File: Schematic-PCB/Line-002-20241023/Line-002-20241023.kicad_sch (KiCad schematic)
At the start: 208 parts

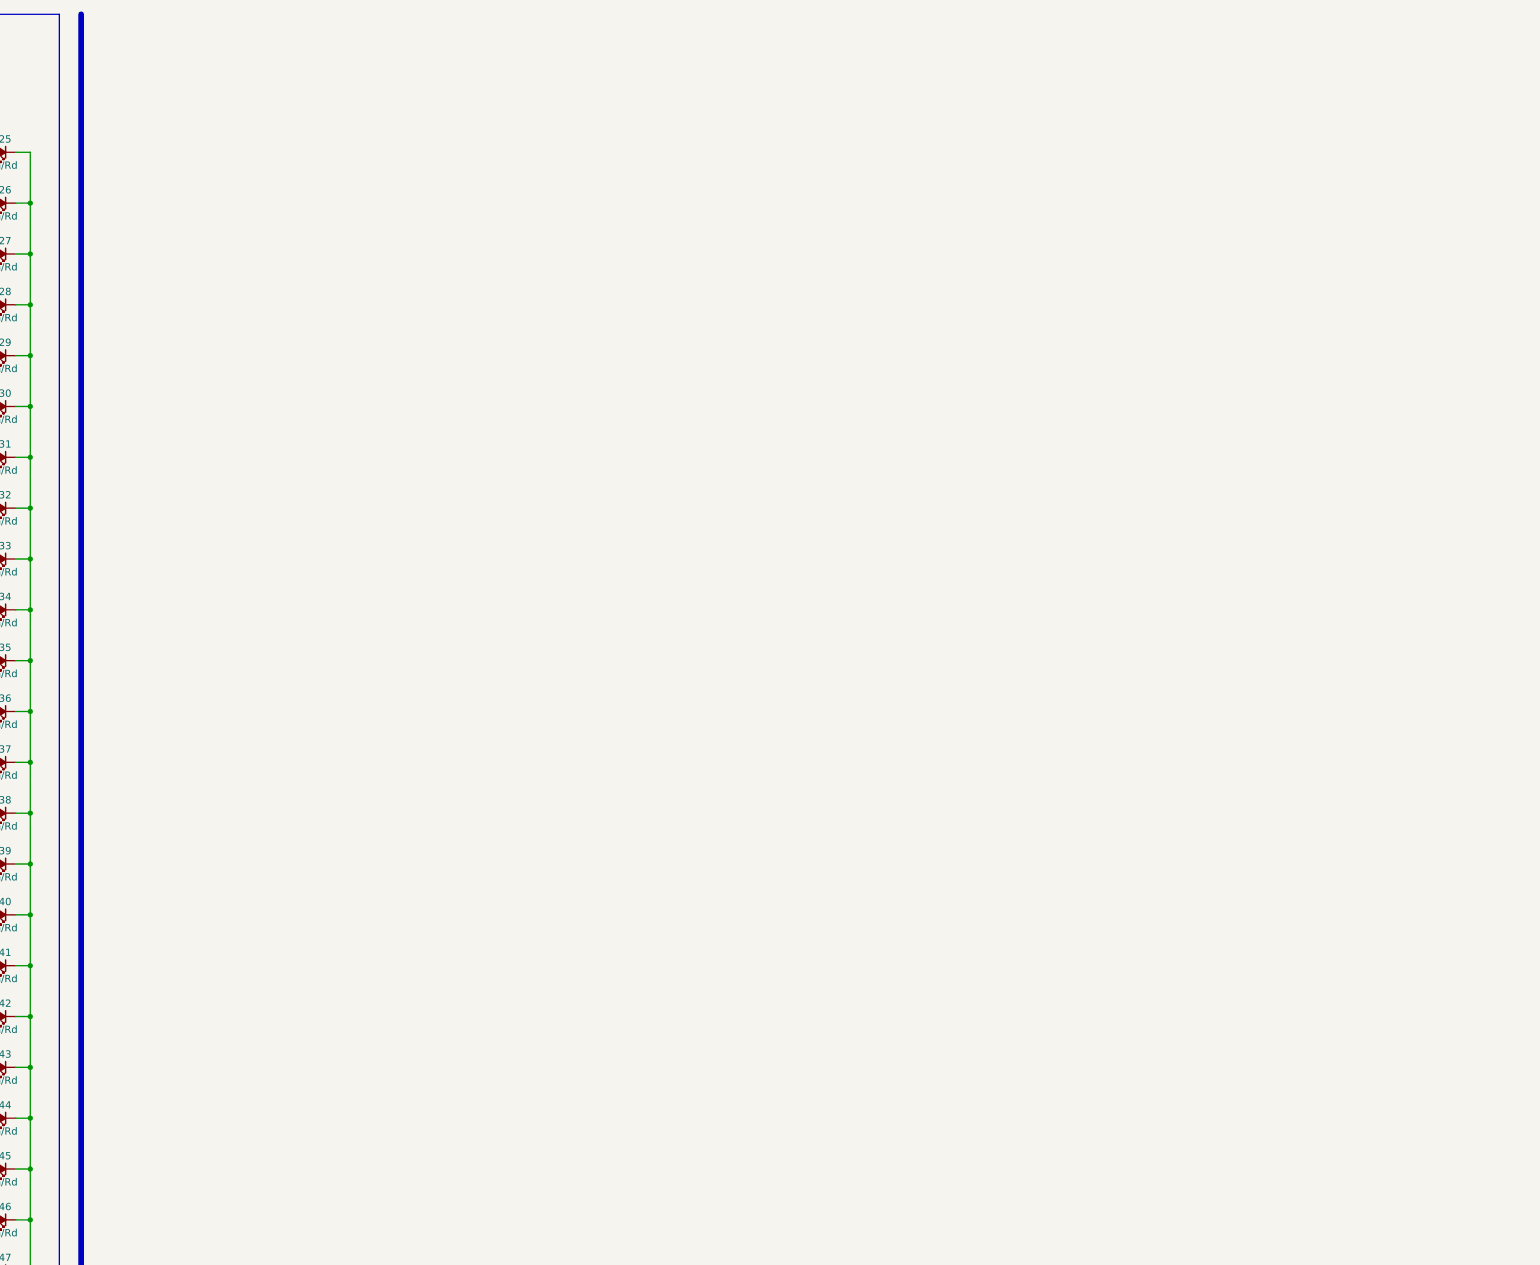
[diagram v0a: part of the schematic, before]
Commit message: update: ラインセンサ基板ver.002を更新した
回路図をちょっと進めた ∧ PCBをやり始めた
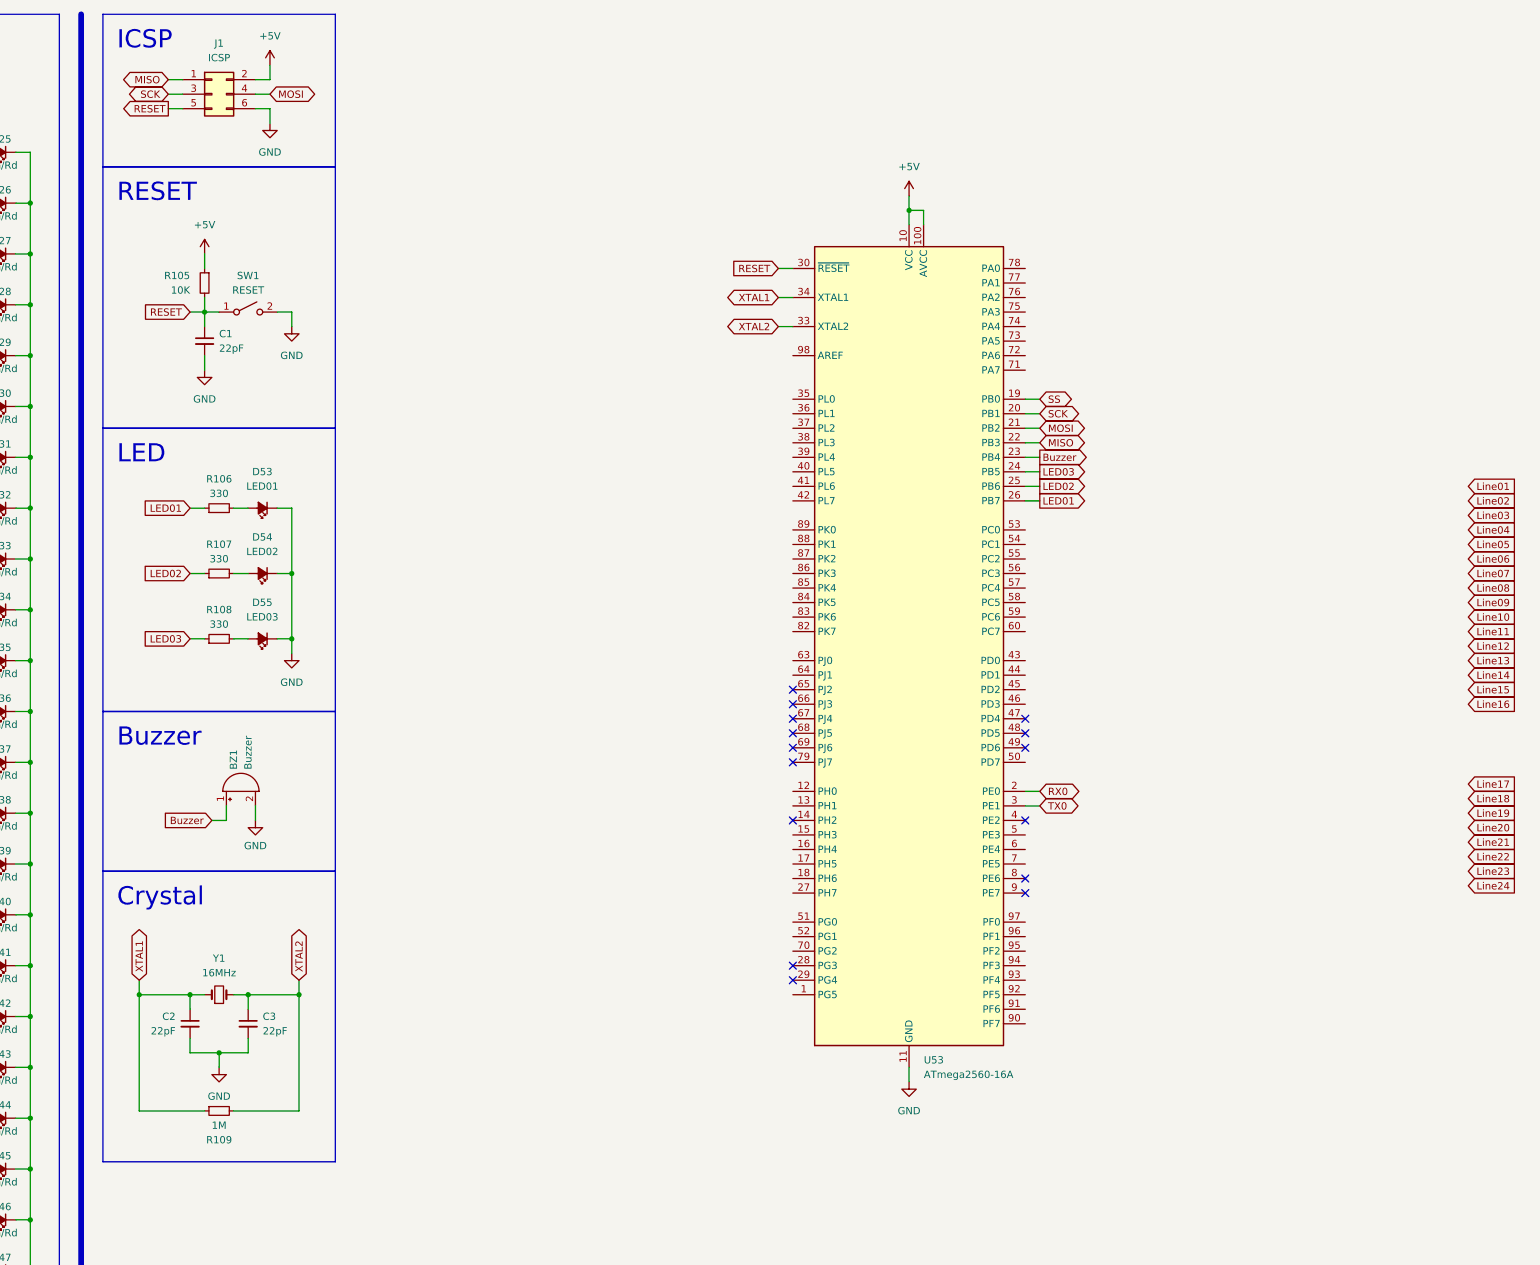
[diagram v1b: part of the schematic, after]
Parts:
- added BZ1: Buzzer, @2024TOINIOT2-Line:PKM13EPYH4000-A0, symbol Device:Buzzer
- added C1, C2, C3: 22pF, symbol Device:C_Small
- added D53: LED01, LED_SMD:LED_0603_1608Metric, symbol Device:LED_Small_Filled
- added D54: LED02, LED_SMD:LED_0603_1608Metric, symbol Device:LED_Small_Filled
- added D55: LED03, LED_SMD:LED_0603_1608Metric, symbol Device:LED_Small_Filled
- added J1: ICSP, symbol Connector_Generic:Conn_02x03_Odd_Even
- added R105: 10K, Resistor_SMD:R_0603_1608Metric, symbol Device:R_Small
- added R106, R107, R108: 330, Resistor_SMD:R_0603_1608Metric, symbol Device:R_Small
- added R109: 1M, symbol Device:R_Small
- added SW1: RESET, symbol Switch:SW_SPST
- added U53: ATmega2560-16A, Package_QFP:TQFP-100_14x14mm_P0.5mm, symbol MCU_Microchip_ATmega:ATmega2560-16A
- added Y1: 16MHz, symbol Device:Crystal_Small
- D1, D10, D11, D12, D13, D14, D15, D16, D17, D18, D19, D2, D20, D21, D22, D23, D24, D25, D26, D27, D28, D29, D3, D30, D31, D32, D33, D34, D35, D36, D37, D38, D39, D4, D40, D41, D42, D43, D44, D45, D46, D47, D48, D49, D5, D50, D51, D52, D6, D7, D8, D9: footprint (none) -> @2024TOINIOT2-Line:LED-3mm
- R1, R10, R100, R101, R102, R103, R104, R11, R12, R13, R14, R15, R16, R17, R18, R19, R2, R20, R21, R22, R23, R24, R25, R26, R27, R28, R29, R3, R30, R31, R32, R33, R34, R35, R36, R37, R38, R39, R4, R40, R41, R42, R43, R44, R45, R46, R47, R48, R49, R5, R50, R51, R52, R53, R54, R55, R56, R57, R58, R59, R6, R60, R61, R62, R63, R64, R65, R66, R67, R68, R69, R7, R70, R71, R72, R73, R74, R75, R76, R77, R78, R79, R8, R80, R81, R82, R83, R84, R85, R86, R87, R88, R89, R9, R90, R91, R92, R93, R94, R95, R96, R97, R98, R99: footprint (none) -> Resistor_SMD:R_0603_1608Metric
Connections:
- net +5V: now also J1.2 (Pin_2), R105.1, U53.10 (VCC), U53.100 (AVCC), U53.31 (VCC), U53.61 (VCC), U53.80 (VCC)
- net GND: now also BZ1.2 (-), C1.2, C2.2, C3.2, D53.1 (K), D54.1 (K), D55.1 (K), J1.6 (Pin_6), SW1.2 (B), U53.11 (GND), U53.32 (GND), U53.62 (GND), U53.81 (GND), U53.99 (GND)
- new net: D53.2 (A), R106.2
- new net: D54.2 (A), R107.2
- new net: D55.2 (A), R108.2
- new net Buzzer: BZ1.1 (+), U53.23 (PB4)
- new net LED01: R106.1, U53.26 (PB7)
- new net LED02: R107.1, U53.25 (PB6)
- new net LED03: R108.1, U53.24 (PB5)
- new net MISO: J1.1 (Pin_1), U53.22 (PB3)
- new net MOSI: J1.4 (Pin_4), U53.21 (PB2)
- new net RESET: C1.1, J1.5 (Pin_5), R105.2, SW1.1 (A), U53.30 (~{RESET})
- new net RX0: U53.2 (PE0)
- new net SCK: J1.3 (Pin_3), U53.20 (PB1)
- new net SS: U53.19 (PB0)
- new net TX0: U53.3 (PE1)
- new net XTAL1: C2.1, R109.1, U53.34 (XTAL1), Y1.1
- new net XTAL2: C3.1, R109.2, U53.33 (XTAL2), Y1.2
- no-connect marks 0 -> 15
